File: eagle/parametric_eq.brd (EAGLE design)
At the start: 100 x 80 mm, 39 parts, among them IC1 TL072P, IC2 TL072P

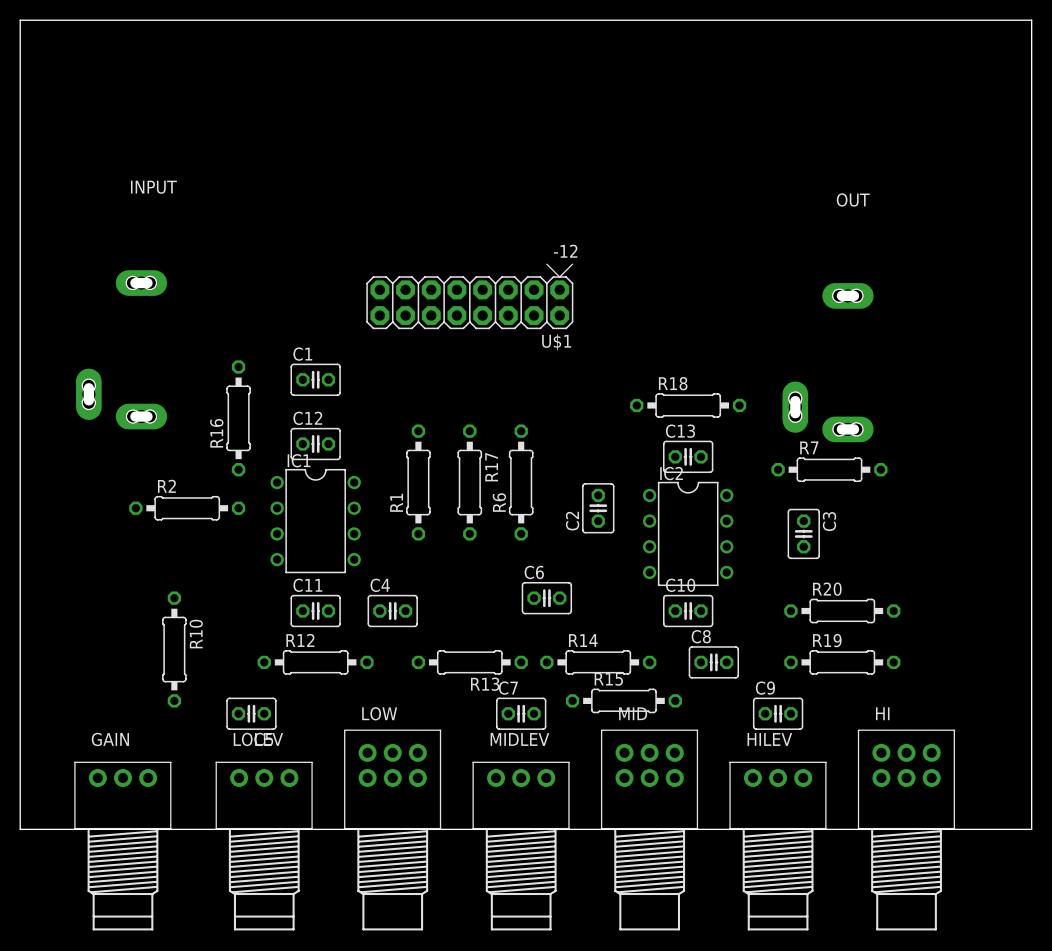
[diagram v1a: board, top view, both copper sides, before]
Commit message: almost routed
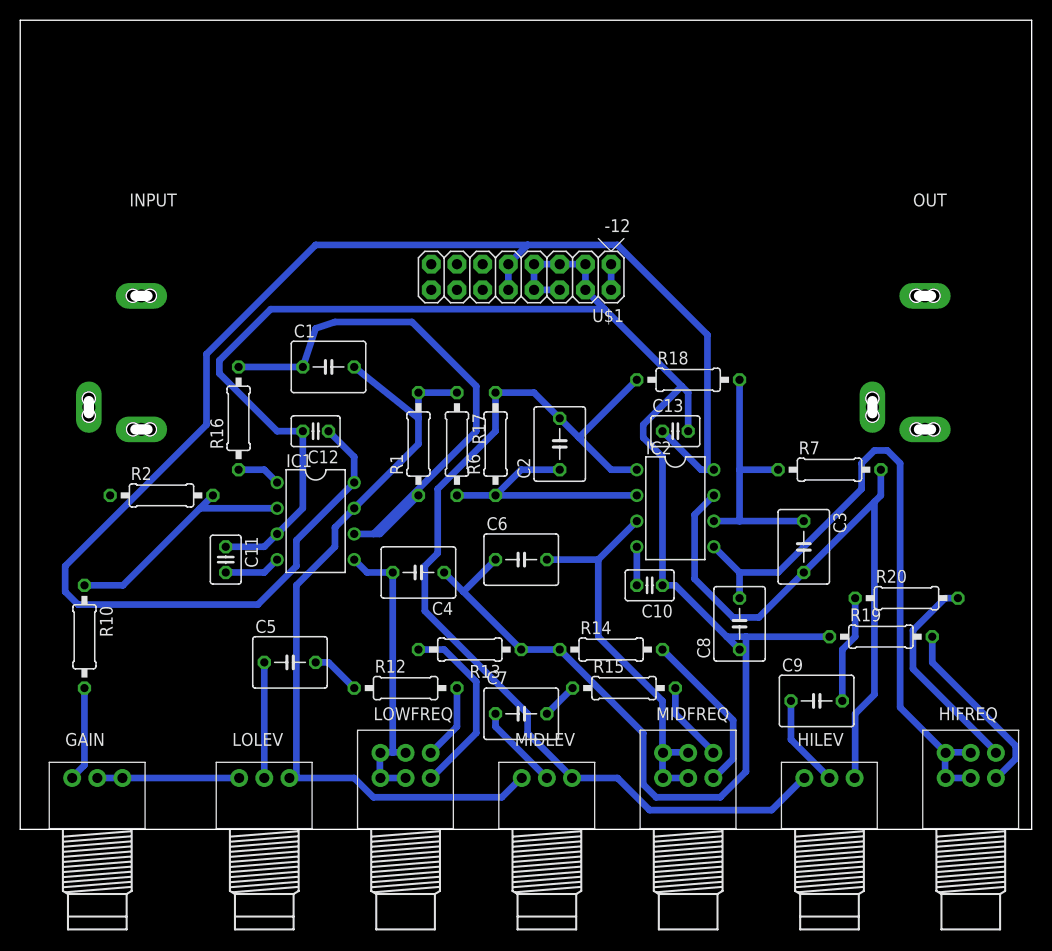
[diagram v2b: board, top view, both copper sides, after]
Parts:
- removed HI, LOW, MID: 50k log, bourns_ptd:PTD902
- added HIFREQ, LOWFREQ, MIDFREQ: 50k log, bourns_ptd:PTD902
- C1, C2, C3, C4, C5, C6, C7, C8, C9: device rcl:C025-030X050 -> rcl:C050-050X075
- moved C11 10.2 mm to (20.3, 26.7), turned to 270 degrees
- moved R12 9.25 mm to (38.1, 14.0)
- moved R10 8.98 mm to (6.35, 19.1)
- moved OUT 7.62 mm to (84.5, 55.2)
- moved C2 7.41 mm to (53.3, 38.1)
- moved R20 6.48 mm to (87.6, 22.9)
- moved C5 6.35 mm to (26.7, 16.5), turned to 0 degrees
- moved U$1 5.68 mm to (52.1, 54.6)
- moved HILEV 5.08 mm to (80.0, 5.08)
- moved C10 4.58 mm to (62.2, 24.1), turned to 180 degrees
- moved C6 4.58 mm to (49.5, 26.7)
- moved R19 4.58 mm to (85.1, 19.1)
- moved R6 4.58 mm to (47.0, 38.1)
- moved C8 4.58 mm to (71.1, 20.3), turned to 90 degrees
- moved C4 4.58 mm to (39.4, 25.4), turned to 180 degrees
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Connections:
- net N$10: now also LOWFREQ.1-3; no longer LOW.1-3
- net N$12: now also LOWFREQ.2-3; no longer LOW.2-3
- net N$16: now also MIDFREQ.2-3; no longer MID.2-3
- net N$17: now also MIDFREQ.1-3; no longer MID.1-3
- net N$18: now also HIFREQ.1-3; no longer HI.1-3
- net N$19: now also HIFREQ.2-3; no longer HI.2-3
- net N$22: now also LOWFREQ.1-1, LOWFREQ.1-2, LOWFREQ.2-1, LOWFREQ.2-2; no longer LOW.1-1, LOW.1-2, LOW.2-1, LOW.2-2
- net N$27: now also MIDFREQ.1-1, MIDFREQ.1-2, MIDFREQ.2-1, MIDFREQ.2-2; no longer MID.1-1, MID.1-2, MID.2-1, MID.2-2
- net N$28: now also HIFREQ.1-1, HIFREQ.1-2, HIFREQ.2-1, HIFREQ.2-2; no longer HI.1-1, HI.1-2, HI.2-1, HI.2-2
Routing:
- net GND: track 0.00 -> 203.2 mm
- net +12V: track 0.00 -> 153.9 mm
- net N$7: track 0.00 -> 97.9 mm
- net N$6: track 0.00 -> 79.6 mm
- net N$28: track 0.00 -> 67.1 mm
- net N$8: track 0.00 -> 64.7 mm
- net N$5: track 0.00 -> 55.7 mm
- net N$27: track 0.00 -> 39.8 mm
- net N$22: track 0.00 -> 29.7 mm
- net N$4: track 0.00 -> 26.7 mm
- net N$3: track 0.00 -> 25.2 mm
- net N$1: track 0.00 -> 24.0 mm
- net N$19: track 0.00 -> 21.3 mm
- net N$10: track 0.00 -> 18.5 mm
- net N$23: track 0.00 -> 18.4 mm
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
